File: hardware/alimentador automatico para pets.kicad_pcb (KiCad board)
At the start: 2 copper layers, 1 part, among them U1 ESP32-DEVKIT-V1

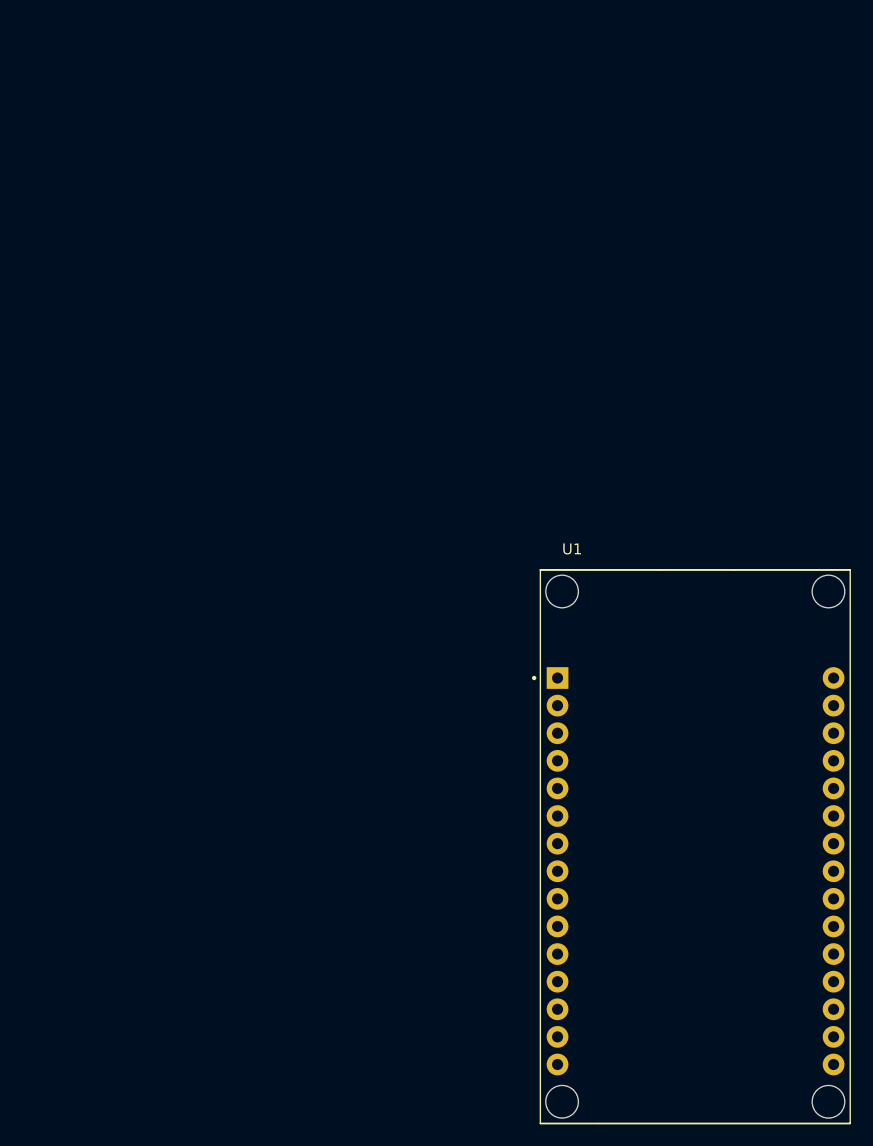
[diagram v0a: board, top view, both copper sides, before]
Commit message: pcb design start
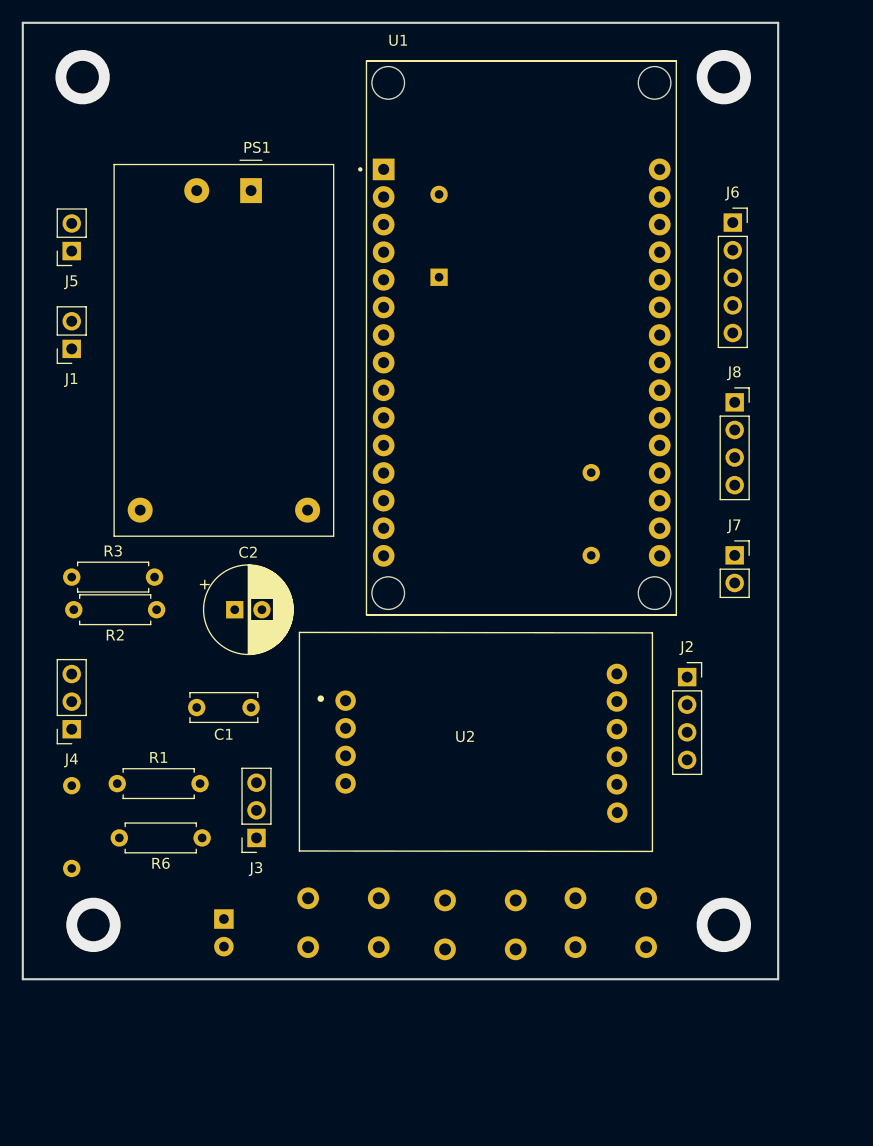
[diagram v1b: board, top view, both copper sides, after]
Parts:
- added C1: 100n, Capacitor_THT:C_Disc_D6.0mm_W2.5mm_P5.00mm, F.Cu at (94.5, 80.0)
- added C2: 220u, Capacitor_THT:CP_Radial_D8.0mm_P2.50mm, F.Cu at (93.0, 71.0)
- added D1: LED, LED_THT:LED_D3.0mm, B.Cu at (92.0, 99.5)
- added D2: 3V6, Diode_THT:D_DO-35_SOD27_P7.62mm_Horizontal, B.Cu at (111.8, 40.4)
- added J1: Conn_01x02, Connector_PinSocket_2.54mm:PinSocket_1x02_P2.54mm_Vertical, F.Cu at (78.0, 47.0)
- added J2: Conn_01x04, Connector_PinSocket_2.54mm:PinSocket_1x04_P2.54mm_Vertical, F.Cu at (134.6, 77.2)
- added J3: Conn_01x03, Connector_PinSocket_2.54mm:PinSocket_1x03_P2.54mm_Vertical, F.Cu at (95.0, 92.0)
- added J4: Conn_01x03, Connector_PinSocket_2.54mm:PinSocket_1x03_P2.54mm_Vertical, F.Cu at (78.0, 82.0)
- added J5: Conn_01x02, Connector_PinSocket_2.54mm:PinSocket_1x02_P2.54mm_Vertical, F.Cu at (78.0, 38.0)
- added J6: Conn_01x05, Connector_PinSocket_2.54mm:PinSocket_1x05_P2.54mm_Vertical, F.Cu at (138.8, 35.4)
- added J7: Conn_01x02, Connector_PinSocket_2.54mm:PinSocket_1x02_P2.54mm_Vertical, F.Cu at (139.0, 66.0)
- added J8: Conn_01x04, Connector_PinSocket_2.54mm:PinSocket_1x04_P2.54mm_Vertical, F.Cu at (139.0, 51.9)
- added PS1: HLK-PM01 5V, Converter_ACDC:Converter_ACDC_HiLink_HLK-PMxx, F.Cu at (94.5, 32.4)
- added R1: 10k, Resistor_THT:R_Axial_DIN0207_L6.3mm_D2.5mm_P7.62mm_Horizontal, F.Cu at (82.2, 87.0)
- added R2: 10k, Resistor_THT:R_Axial_DIN0207_L6.3mm_D2.5mm_P7.62mm_Horizontal, F.Cu at (85.8, 71.0)
- added R3: 4k7, Resistor_THT:R_Axial_DIN0207_L6.3mm_D2.5mm_P7.62mm_Horizontal, F.Cu at (78.0, 68.0)
- added R4: 470, Resistor_THT:R_Axial_DIN0207_L6.3mm_D2.5mm_P7.62mm_Horizontal, B.Cu at (78.0, 87.2)
- added R5: 470, Resistor_THT:R_Axial_DIN0207_L6.3mm_D2.5mm_P7.62mm_Horizontal, B.Cu at (125.8, 58.4)
- added R6: 10k, Resistor_THT:R_Axial_DIN0207_L6.3mm_D2.5mm_P7.62mm_Horizontal, F.Cu at (90.0, 92.0)
- added SW1: SW_Push, Button_Switch_THT:SW_PUSH_6mm, B.Cu at (118.8, 97.8)
- added SW2: SW_Push, Button_Switch_THT:SW_PUSH_6mm, B.Cu at (130.8, 97.5)
- added SW3: SW_Push, Button_Switch_THT:SW_PUSH_6mm, B.Cu at (106.2, 97.5)
- added U2: HX711_module, footprint_lib:HX711_module, F.Cu at (114.2, 83.2)
- moved U1 49.5 mm to (119.4, 46.0)
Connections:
- net Net-(U1-Pad2) renamed GND
- U1 pad 1: unconnected-(U1-Pad1) -> /3V3
- U1 pad 10: unconnected-(U1-Pad10) -> /sMotor
- U1 pad 11: unconnected-(U1-Pad11) -> /SDA_disp
- U1 pad 14: unconnected-(U1-Pad14) -> /SCL_disp
- U1 pad 19: unconnected-(U1-Pad19) -> /led_on
- U1 pad 21: unconnected-(U1-Pad21) -> /BUTTON_1
- U1 pad 22: unconnected-(U1-Pad22) -> /BUTTON_2
- U1 pad 23: unconnected-(U1-Pad23) -> /BUTTON_3
- U1 pad 25: unconnected-(U1-Pad25) -> /SCK
- U1 pad 26: unconnected-(U1-Pad26) -> /DT_encoder
- U1 pad 27: unconnected-(U1-Pad27) -> /DT
- U1 pad 28: unconnected-(U1-Pad28) -> /SW_encoder
- U1 pad 3: unconnected-(U1-Pad3) -> /CLK_encoder
- U1 pad 30: unconnected-(U1-Pad30) -> /5V
- U1 pad 5: unconnected-(U1-Pad5) -> /IR_out
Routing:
- net GND: vias 0 -> 4
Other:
- board outline added: 69.5 x 88 mm
